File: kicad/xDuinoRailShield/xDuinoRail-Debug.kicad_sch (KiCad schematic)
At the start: 0 parts

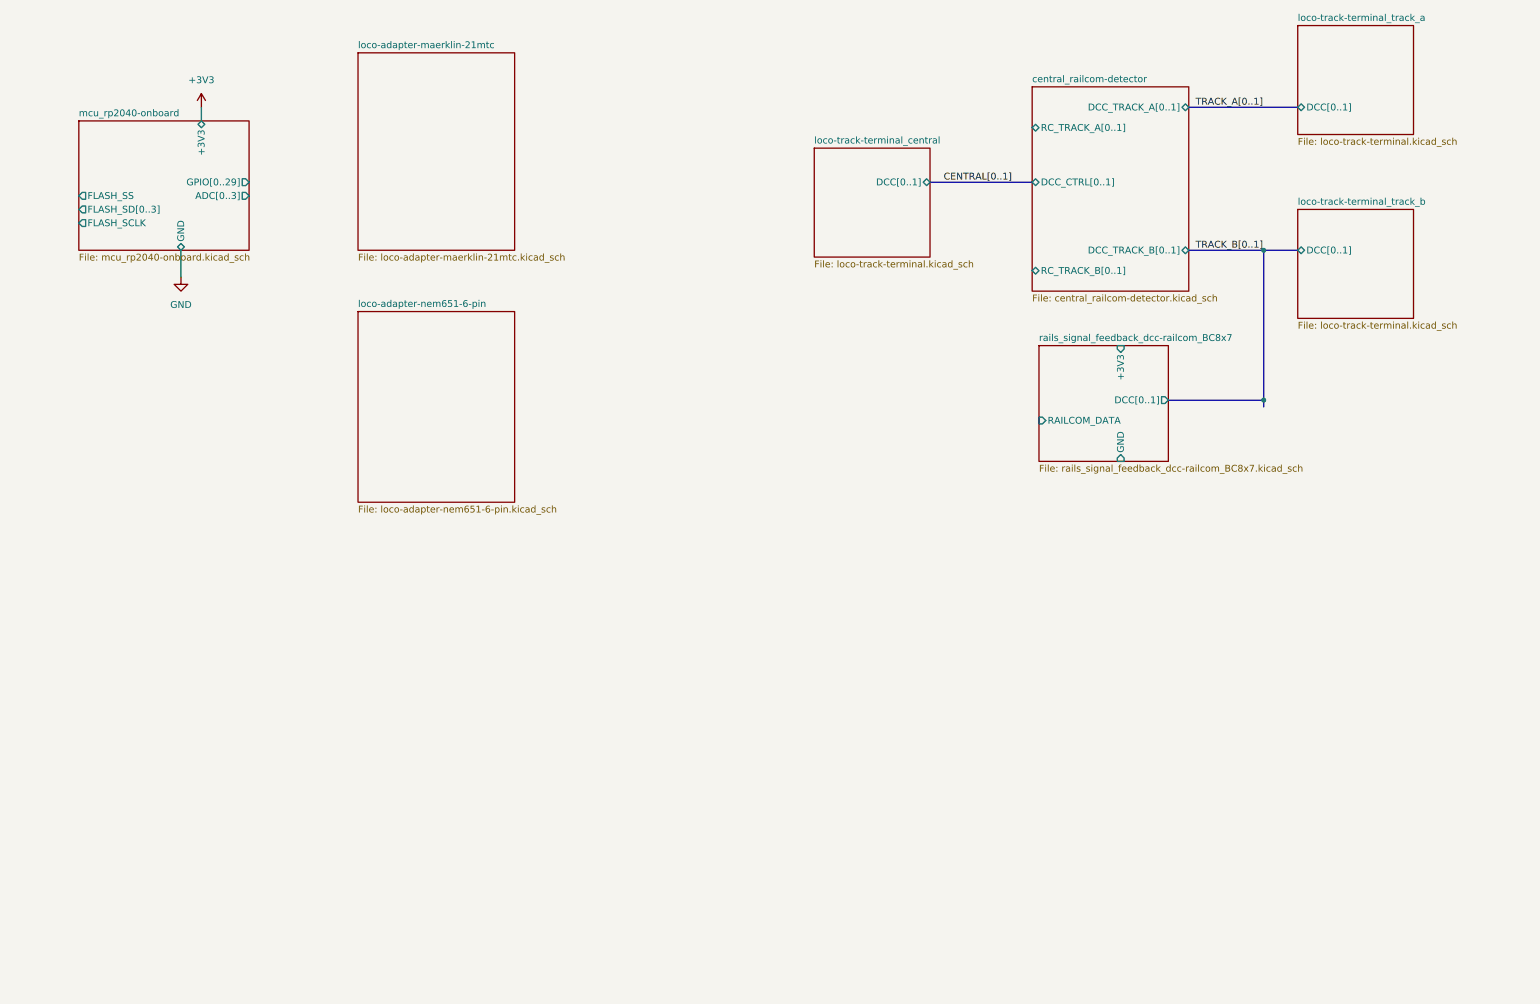
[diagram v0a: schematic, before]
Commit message: More stuff
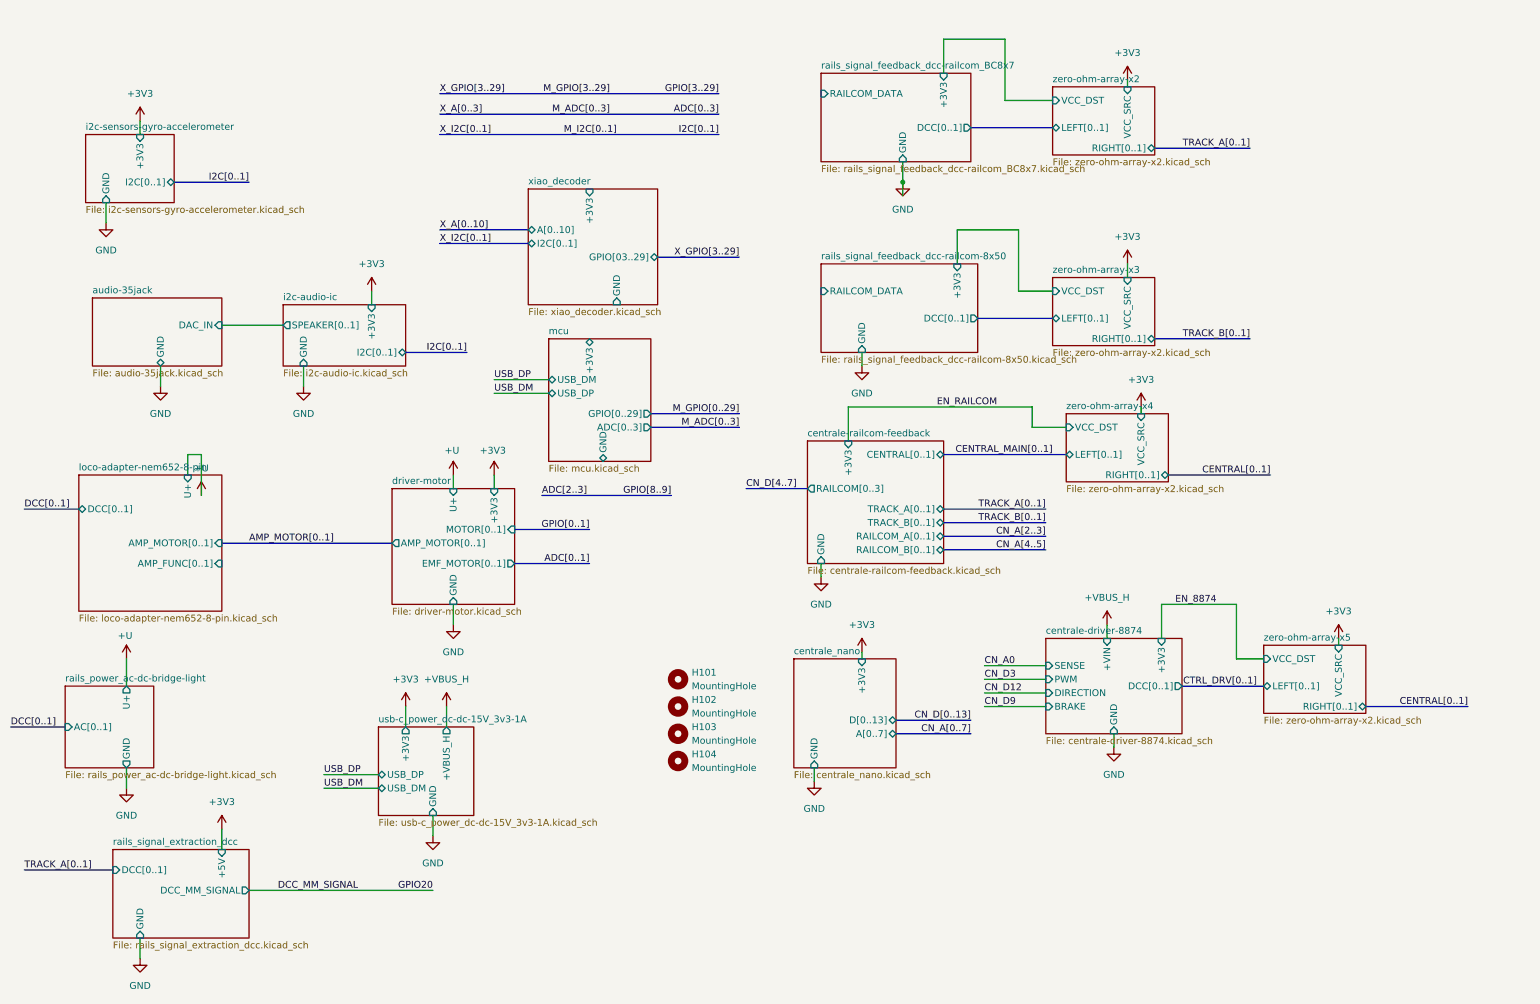
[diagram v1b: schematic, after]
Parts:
- added H101, H102, H103, H104: MountingHole, MountingHole:MountingHole_2.2mm_M2, symbol Mechanical:MountingHole
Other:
- removed sheet central_railcom-detector
- removed sheet loco-adapter-maerklin-21mtc
- removed sheet loco-adapter-nem651-6-pin
- removed sheet loco-track-terminal_central
- removed sheet loco-track-terminal_track_a
- removed sheet loco-track-terminal_track_b
- removed sheet mcu_rp2040-onboard
- added sheet audio-35jack (audio-35jack.kicad_sch)
- added sheet centrale-driver-8874 (centrale-driver-8874.kicad_sch)
- added sheet centrale-railcom-feedback (centrale-railcom-feedback.kicad_sch)
- added sheet centrale_nano (centrale_nano.kicad_sch)
- added sheet driver-motor (driver-motor.kicad_sch)
- added sheet i2c-audio-ic (i2c-audio-ic.kicad_sch)
- added sheet i2c-sensors-gyro-accelerometer (i2c-sensors-gyro-accelerometer.kicad_sch)
- added sheet loco-adapter-nem652-8-pin (loco-adapter-nem652-8-pin.kicad_sch)
- added sheet mcu (mcu.kicad_sch)
- added sheet rails_power_ac-dc-bridge-light (rails_power_ac-dc-bridge-light.kicad_sch)
- added sheet rails_signal_extraction_dcc (rails_signal_extraction_dcc.kicad_sch)
- added sheet rails_signal_feedback_dcc-railcom-8x50 (rails_signal_feedback_dcc-railcom-8x50.kicad_sch)
- added sheet usb-c_power_dc-dc-15V_3v3-1A (usb-c_power_dc-dc-15V_3v3-1A.kicad_sch)
- added sheet xiao_decoder (xiao_decoder.kicad_sch)
- added sheet zero-ohm-array-x2 (zero-ohm-array-x2.kicad_sch)
- added sheet zero-ohm-array-x3 (zero-ohm-array-x2.kicad_sch)
- added sheet zero-ohm-array-x4 (zero-ohm-array-x2.kicad_sch)
- added sheet zero-ohm-array-x5 (zero-ohm-array-x2.kicad_sch)
